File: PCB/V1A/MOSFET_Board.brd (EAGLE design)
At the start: 230 x 115 mm, 278 parts, among them IC301 78L05_TO-220AB-3-BR, IC302 78L05_TO-220AB-3-BR, J301 TEMP, J302 +12V, J303 CTRL, J304 FAN_MOLEX4PIN, J305 FAN_MOLEX4PIN, J306 DUT+, J307 DUT-, Q201 SIRC10DP, Q202 SIRC10DP, Q203 BC817, Q204 BC817, Q205 SIRC10DP, Q206 SIRC10DP, Q207 BC817, Q208 BC807, Q209 BC817, Q210 BC807, Q211 IXTK102N65X2, Q212 IXTK102N65X2, Q301 BC817, Q302 BC817, Q401 BC807, Q402 BC807, Q403 BC807, Q404 BC807, Q405 BC807, Q406 BC807, Q407 BC807, Q408 BC807, Q409 BC807, Q410 BC807, Q411 BC807, Q412 BC807, Q413 BC807, Q414 BC807, U201 AD420, U202 AD420, U203 LT1014I, U204 LT1014I, U205 AD620, U206 AD620, U207 AD620, U208 AD620, U209 LTC1865L, U210 LTC1865L, U301 LP2985-3.1, U302 LP2985-3.1, U303 LP2985-3.1, U304 AD620, U305 LTC1865L, U306 LTC1865L, U307 MAX743, U401 HCPL-063N, U402 HCPL-063N, U403 HCPL-063N, U404 HCPL-063N, U405 HCPL-063N, U406 HCPL-063N, U407 HCPL-063N

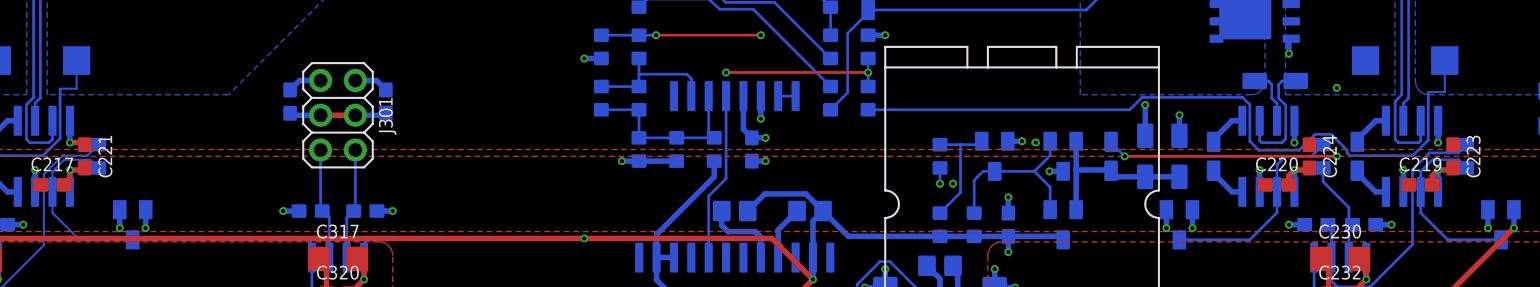
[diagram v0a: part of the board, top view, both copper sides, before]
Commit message: PCB layout
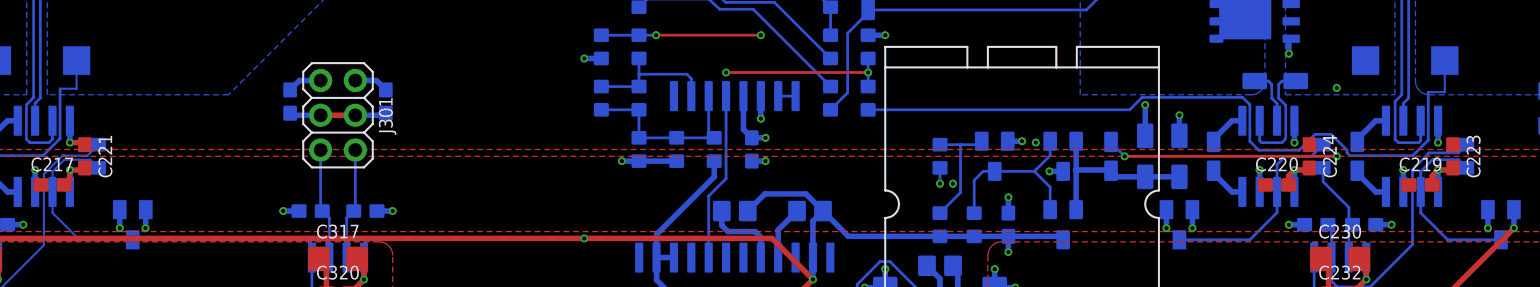
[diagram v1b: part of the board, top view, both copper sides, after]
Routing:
- net -15V: track 115.7 -> 114.4 mm
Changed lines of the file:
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@@
 <layer number="13" name="Route13" color="21" fill="1" visible="no" active="no"/>
 <layer number="14" name="Route14" color="22" fill="1" visible="no" active="no"/>
-<layer number="15" name="Route15" color="23" fill="1" visible="no" active="yes"/>
+<layer number="15" name="Route15" color="23" fill="1" visible="yes" active="yes"/>
 <layer number="16" name="Bottom" color="1" fill="1" visible="yes" active="yes"/>
 <layer number="17" name="Pads" color="2" fill="1" visible="yes" active="yes"/>
@@
 <via x="-19.595" y="8" extent="1-16" drill="0.3" diameter="0.6"/>
 <wire x1="80.405" y1="9.6" x2="80.405" y2="8" width="0.4064" layer="16"/>
-<wire x1="81.5" y1="7.85" x2="81.35" y2="8" width="0.4064" layer="1"/>
 <via x="69.905" y="8" extent="1-16" drill="0.3" diameter="0.6"/>
-<wire x1="70" y1="8" x2="69.905" y2="8" width="0.4064" layer="1"/>
-<wire x1="70.85" y1="8" x2="71" y2="7.85" width="0.4064" layer="1"/>
 <wire x1="69.905" y1="9.6" x2="69.905" y2="8" width="0.4064" layer="16"/>
-<wire x1="71" y1="7.85" x2="71.15" y2="8" width="0.4064" layer="1"/>
 <contactref element="Q301" pad="2"/>
 <via x="96" y="-10.905" extent="1-16" drill="0.3" diameter="0.6"/>
@@
 <wire x1="-18.65" y1="8" x2="-19.595" y2="8" width="0.4064" layer="1"/>
 <wire x1="-28.85" y1="8" x2="-29" y2="7.85" width="0.4064" layer="1"/>
-<wire x1="-18.5" y1="7.85" x2="-18.35" y2="8" width="0.4064" layer="1"/>
-<wire x1="81.65" y1="8" x2="81.5" y2="7.85" width="0.4064" layer="1"/>
 <via x="31.25" y="23.65" extent="1-16" drill="0.3" diameter="0.6"/>
 <wire x1="30" y1="23.65" x2="31.25" y2="23.65" width="0.4064" layer="16"/>
 <wire x1="29.635" y1="20.6" x2="29.635" y2="23.285" width="0.4064" layer="16"/>
 <wire x1="29.635" y1="23.285" x2="30" y2="23.65" width="0.4064" layer="16"/>
-<wire x1="50.8271625" y1="8" x2="51" y2="8" width="0.4064" layer="1"/>
 <via x="52" y="-62.1" extent="1-16" drill="0.3" diameter="0.6"/>
 <wire x1="53.05" y1="-62.1" x2="52" y2="-62.1" width="0.4064" layer="16"/>
